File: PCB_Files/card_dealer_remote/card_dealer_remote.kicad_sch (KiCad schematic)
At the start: 9 parts, among them SW1 SW_Push, U1 TLC555xD

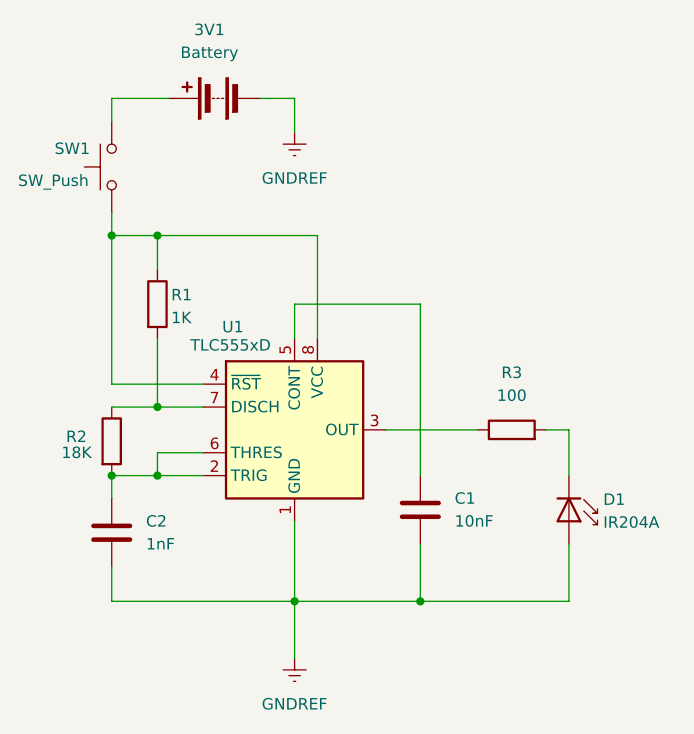
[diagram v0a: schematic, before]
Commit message: Changed the pcb schematics
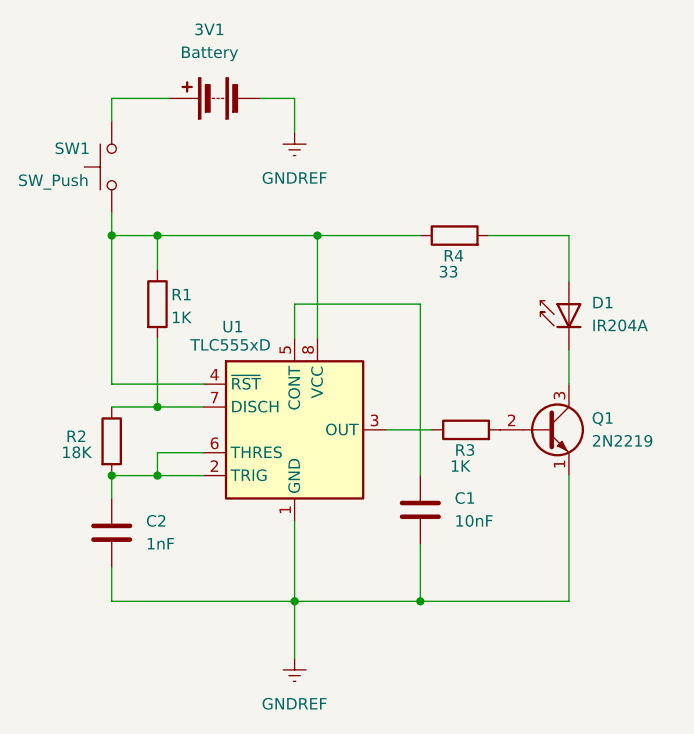
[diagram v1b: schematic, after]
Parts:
- added Q1: 2N2219, Package_TO_SOT_THT:TO-39-3, symbol Transistor_BJT:2N2219
- added R4: 33, Package_DIP:DIP-8_W7.62mm, symbol Device:R
- R3: value 100 -> 1K
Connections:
- net GNDREF: now also Q1.1 (E); no longer D1.2 (A)
- net at D1.1 (K): now also Q1.3 (C); no longer R3.2
- net at R1.1, SW1.1, U1.4 (~{RST})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: now also R4.1
- new net: D1.2 (A), R4.2
- new net: Q1.2 (B), R3.2
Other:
- moved on the sheet: D1
